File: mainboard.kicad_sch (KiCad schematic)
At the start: 19 parts, among them J1 Barrel_Jack, P1 USB_C_Plug_USB2.0, SW1 SW_Push, SW2 SW_Push, U2 ESP32-C3-WROOM-02, U5 LT1963AxST-3.3

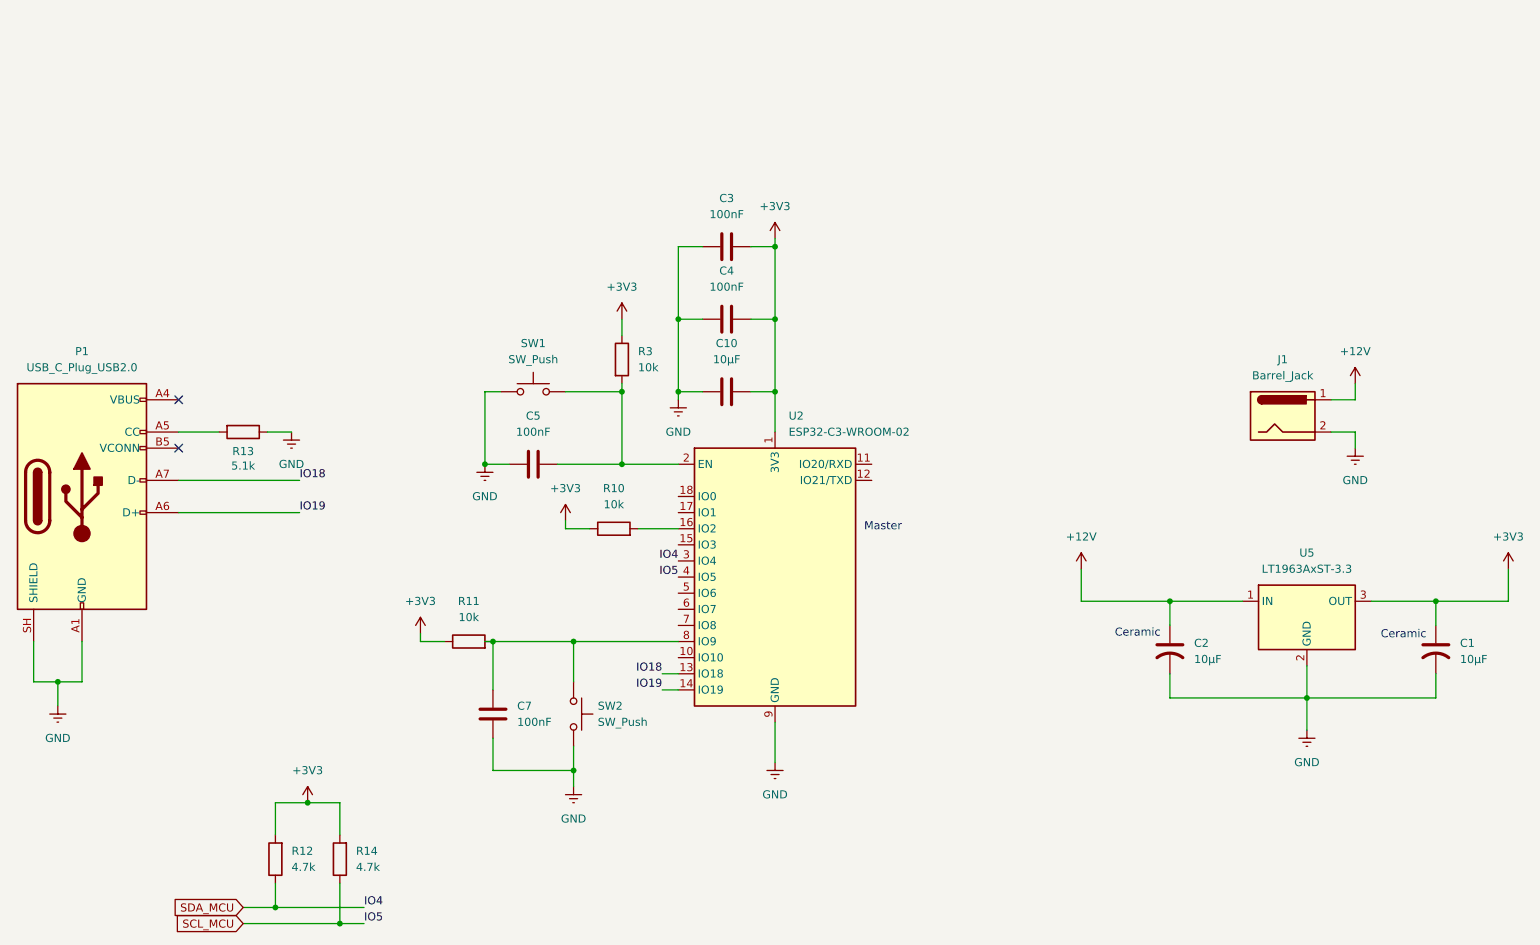
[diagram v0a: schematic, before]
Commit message: Final Design
Pushing it so I can make it into single layer on my PC
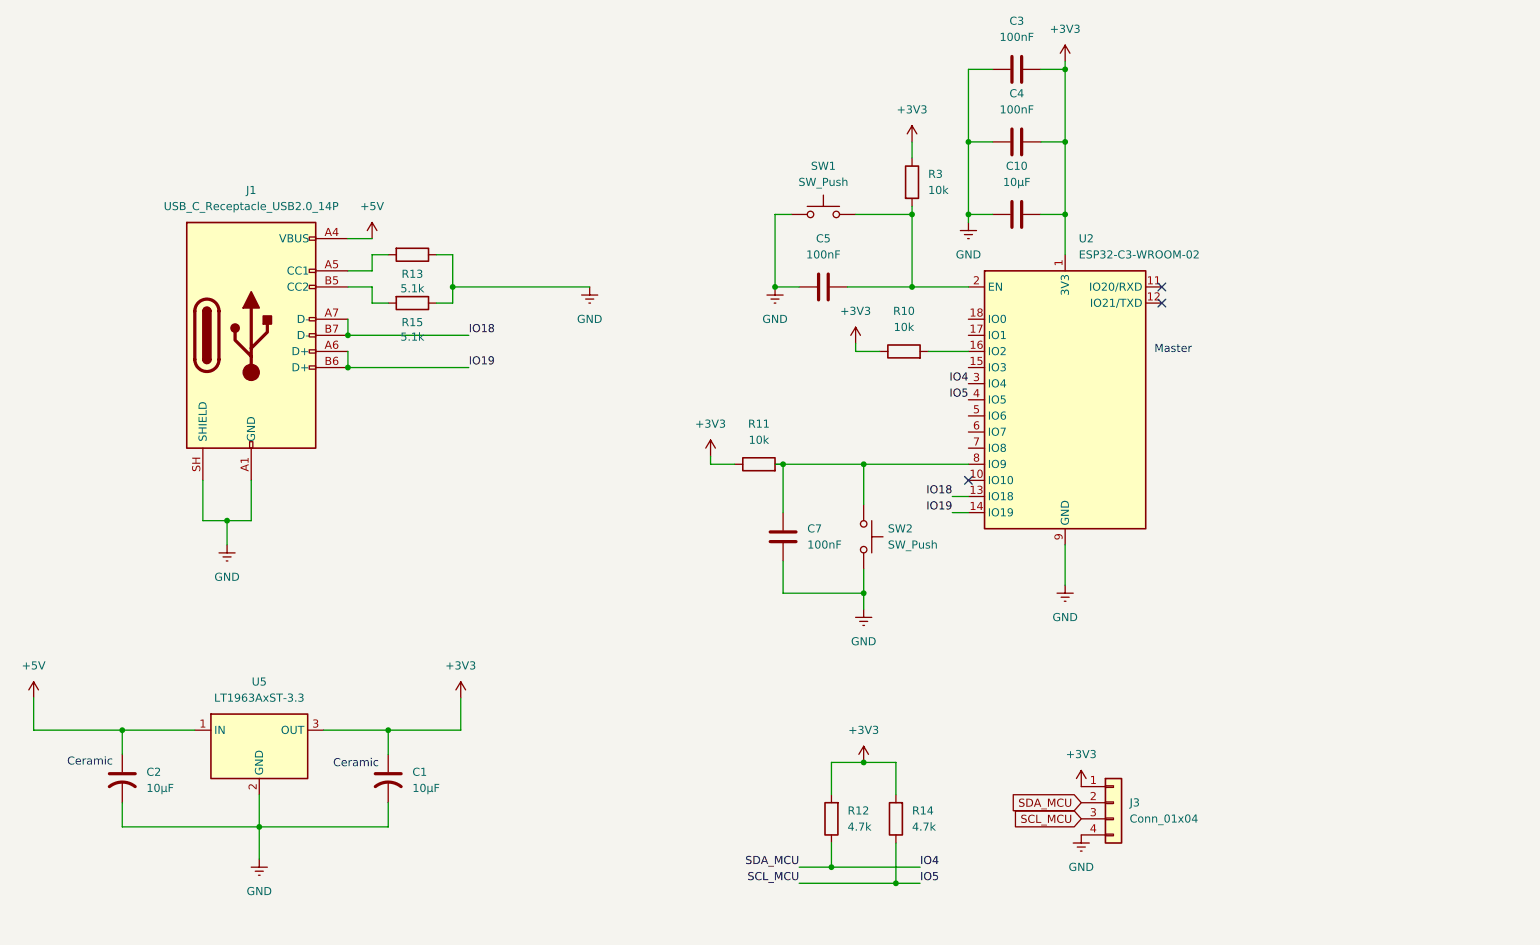
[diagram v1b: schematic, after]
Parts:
- removed J1: Barrel_Jack, Connector_BarrelJack:BarrelJack_Wuerth_6941xx301002, symbol Connector:Barrel_Jack
- removed P1: USB_C_Plug_USB2.0, Connector_USB:USB_C_Receptacle_GCT_USB4105-xx-A_16P_TopMnt_Horizontal, symbol Connector:USB_C_Plug_USB2.0
- added J1: USB_C_Receptacle_USB2.0_14P, symbol Connector:USB_C_Receptacle_USB2.0_14P
- added J3: Conn_01x04, Connector_PinHeader_1.27mm:PinHeader_1x04_P1.27mm_Horizontal, symbol Connector_Generic:Conn_01x04
- added R15: 5.1k, Resistor_SMD:R_0805_2012Metric_Pad1.20x1.40mm_HandSolder, symbol Device:R
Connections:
- net +3V3: now also J3.1 (Pin_1)
- net GND: now also J1.A1 (GND), J1.A12 (GND), J1.B1 (GND), J1.B12 (GND), J1.SH (SHIELD), J3.4 (Pin_4), R15.1
- net IO18: now also J1.A7 (D-), J1.B7 (D-)
- net IO19: now also J1.A6 (D+), J1.B6 (D+)
- net SCL_MCU: now also J3.3 (Pin_3)
- net SDA_MCU: now also J3.2 (Pin_2)
- net at R13.2: now also J1.A5 (CC1)
- net +12V renamed +5V
- net +5V: now also J1.A4 (VBUS), J1.A9 (VBUS), J1.B4 (VBUS), J1.B9 (VBUS)
- new net: J1.B5 (CC2), R15.2
- no-connect marks 2 -> 3
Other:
- moved on the sheet: C1, C10, C2, C3, C4, C5, C7, R10, R11, R12, R14, R3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
